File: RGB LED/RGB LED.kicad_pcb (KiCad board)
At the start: 2 copper layers, 80 x 75 mm, 82 parts, among them J1 USB_C_Receptacle_USB2.0_16P, SW1 SW_SPST_FSMSM, SW2 SW_SPST_FSMSM, U1 AP2112K-3.3, U2 MAX7219, U3 ESP32-S3-WROOM-1-N4

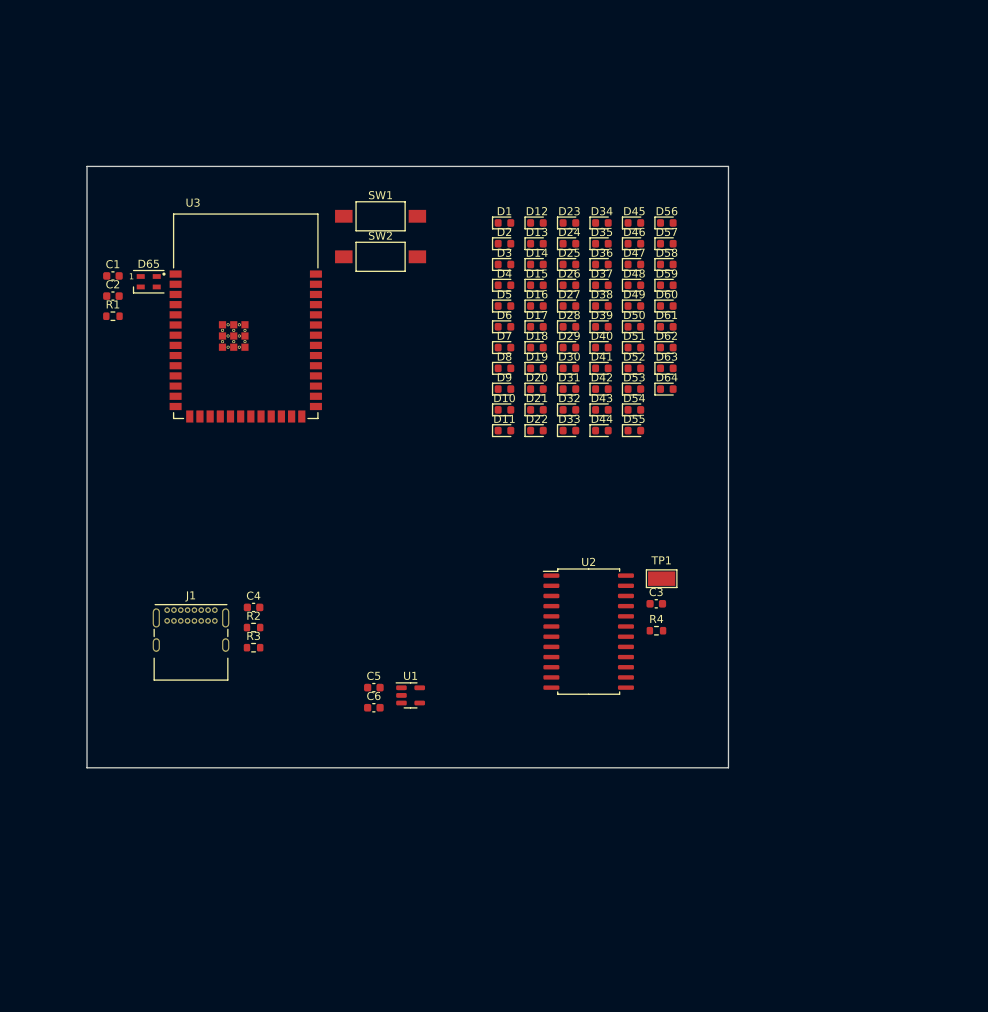
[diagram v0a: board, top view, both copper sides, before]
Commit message: layout update
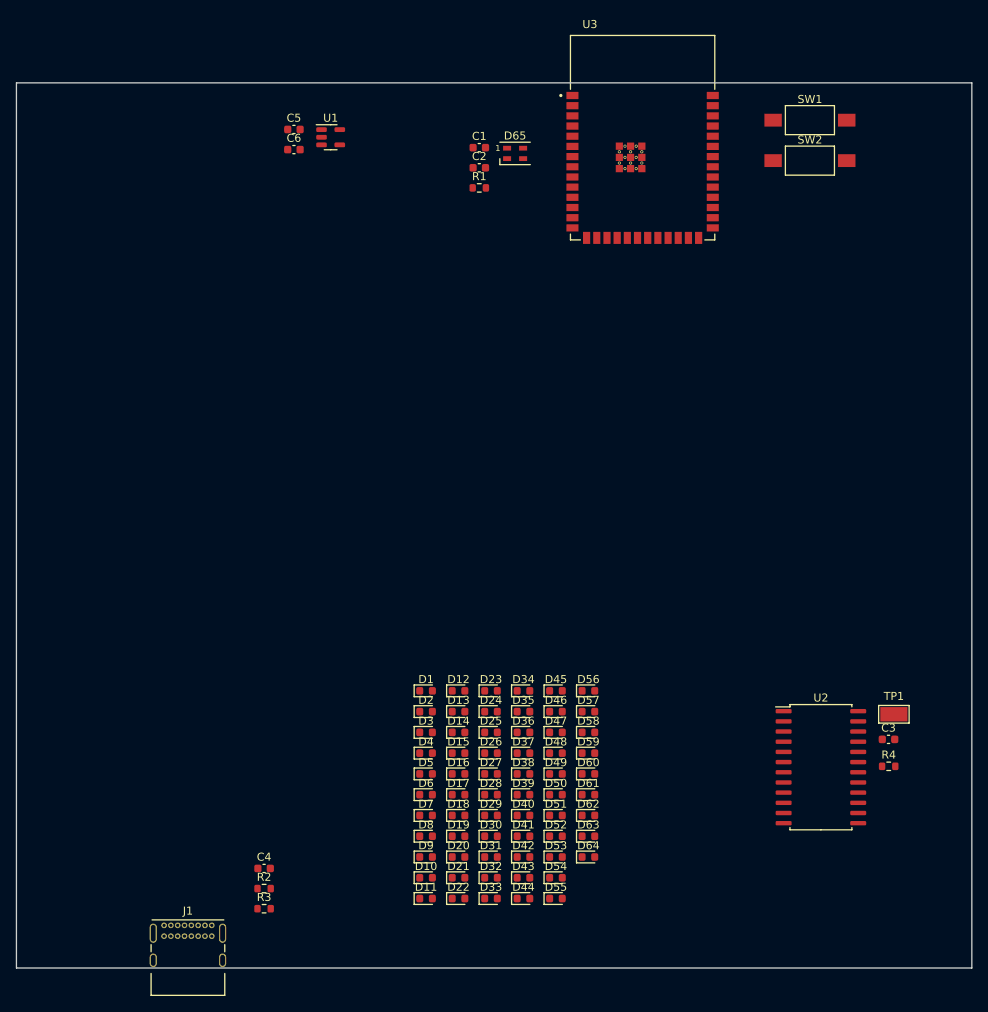
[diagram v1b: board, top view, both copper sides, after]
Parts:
- moved C6 70.3 mm to (75.8, 22.9)
- moved C5 70.3 mm to (75.8, 20.4)
- moved U1 70.3 mm to (80.4, 21.4)
- moved D14 59.2 mm to (96.3, 95.6)
- moved D15 59.2 mm to (96.3, 98.2)
- moved D19 59.2 mm to (96.3, 108.5)
- moved D20 59.2 mm to (96.3, 111.1)
- moved D25 59.2 mm to (100.4, 95.6)
- moved D26 59.2 mm to (100.4, 98.2)
- moved D3 59.2 mm to (92.3, 95.6)
- moved D30 59.2 mm to (100.4, 108.5)
- moved D36 59.2 mm to (104.4, 95.6)
- moved D37 59.2 mm to (104.4, 98.2)
- moved D4 59.2 mm to (92.3, 98.2)
- moved D41 59.2 mm to (104.4, 108.5)
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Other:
- board size 80 x 75 mm -> 119.2 x 110.4 mm
